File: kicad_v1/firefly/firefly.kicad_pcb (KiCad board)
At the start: 2 copper layers, 30.5 x 30.5 mm, 18 parts, among them J1 SEL_CA_CC, J2 ISP, J3 Vin, J4 Vout, Q1 SHF3310, U1 ATtiny13A-P

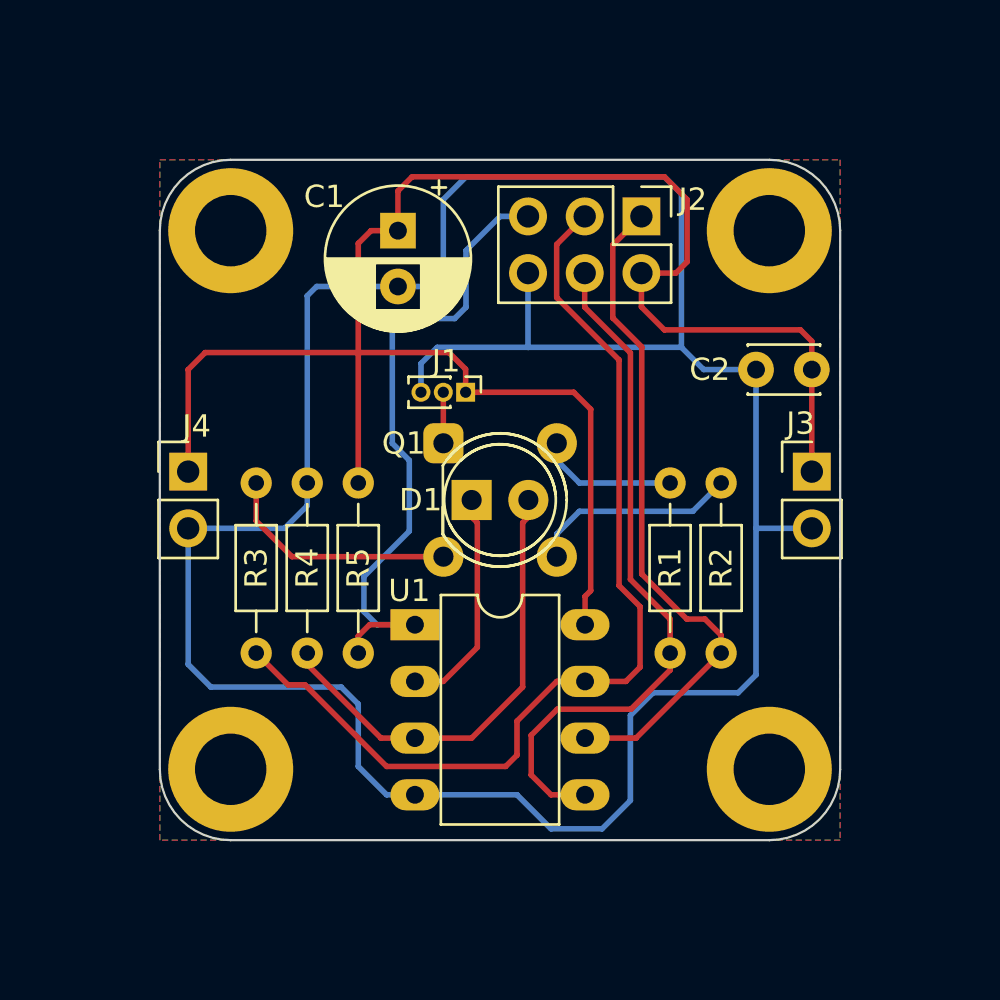
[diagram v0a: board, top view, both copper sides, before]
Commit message: added code
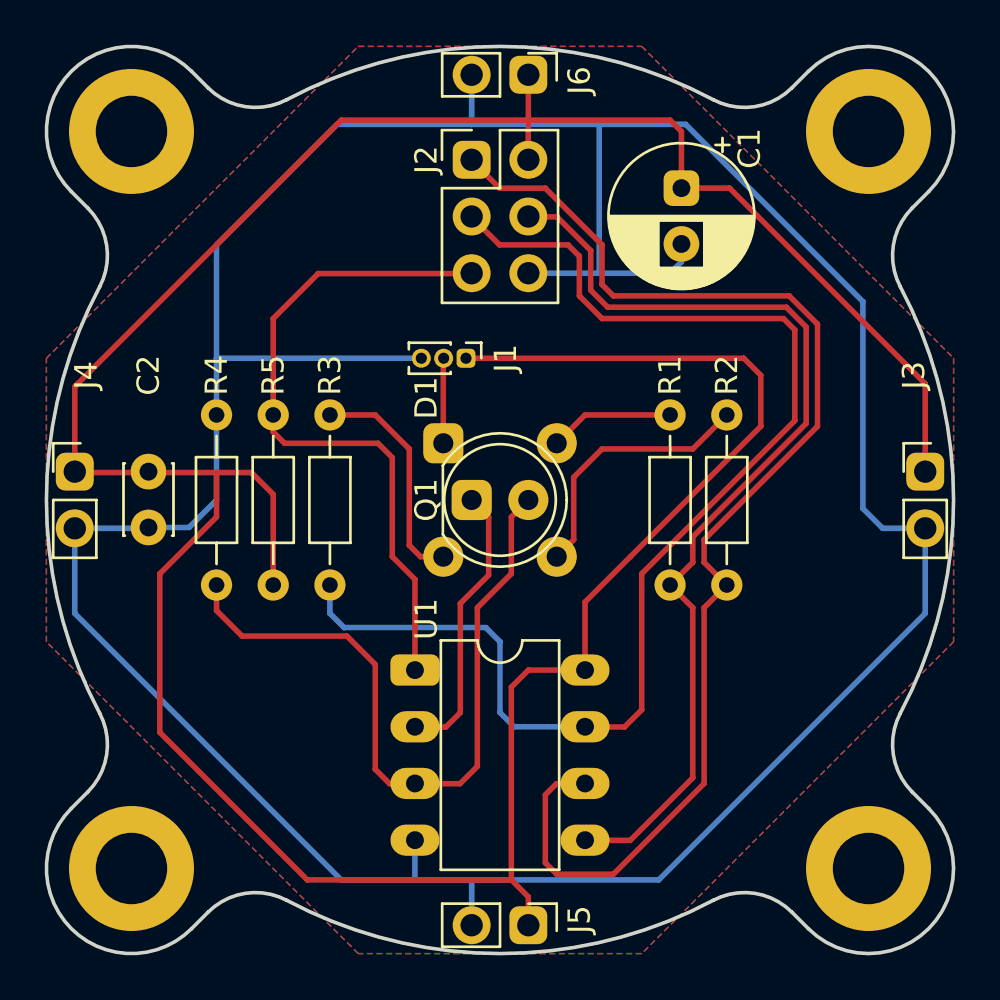
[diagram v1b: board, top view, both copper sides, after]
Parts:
- added J5: Vout, firefly:PinHeader_1x02_P2.54mm_Vertical, F.Cu at (52.1, 69.8)
- added J6: Vout, firefly:PinHeader_1x02_P2.54mm_Vertical, F.Cu at (52.1, 31.8)
- J4: value Vout -> Vin
- moved C2 30.1 mm to (35.1, 49.5), turned to -90 degrees
- moved C1 12.8 mm to (58.9, 36.8)
- moved J2 8.02 mm to (49.5, 35.6), turned to 0 degrees
- moved H1 6.29 mm to (34.3, 34.3)
- moved H2 6.29 mm to (67.3, 34.3)
- moved H3 6.29 mm to (67.3, 67.3)
- moved H4 6.29 mm to (34.3, 67.3)
- moved R5 5.95 mm to (40.6, 54.6), turned to 90 degrees
- moved R4 5.08 mm to (38.1, 54.6)
- moved J3 5.08 mm to (69.8, 49.5)
- moved J4 5.08 mm to (31.8, 49.5)
- moved R3 4.49 mm to (43.2, 54.6)
- moved R2 3.06 mm to (61.0, 54.6)
- moved R1 3.05 mm to (58.4, 54.6)
- moved U1 2.03 mm to (47.0, 58.4)
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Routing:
- net VCC: track 83.2 -> 150.2 mm
- net GND: track 121.1 -> 150.6 mm
- net /MISO: track 30.3 -> 57.2 mm
- net /MOSI: track 31.4 -> 44.7 mm
- net /SCK: track 44.3 -> 57.0 mm
- net /XTAL2: track 21.0 -> 32.0 mm
- net Net-(D1-GK): track 9.33 -> 11.9 mm
- net /XTAL1: track 10.1 -> 12.7 mm
- net Net-(D1-A): track 2.29 -> 3.81 mm
- net /RST: track 29.5 -> 30.6 mm
- net Net-(D1-RK): track 6.26 -> 5.61 mm
- net Net-(D1-BK): track 10.8 -> 10.2 mm
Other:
- board size 30.5 x 30.5 mm -> 40.6 x 40.6 mm
